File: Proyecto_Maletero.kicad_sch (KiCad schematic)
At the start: 47 parts, among them J1 DE9_Pins, J2 Conn_01x02, J3 Conn_01x02, J4 Conn_01x03, J5 Conn_01x02, J6 DE9_Pins, J8 Conn_01x02, J9 Conn_01x02, K1 FINDER-34.51, Q1 NPN, SW1 SW_Push, SW2 SW_Push, U1 LM1084-5.0, U2 MCP2551-I-SN, U3 PIC18F258-I_SO, U4 L298HN, U5 LM321, Y1 4MHz

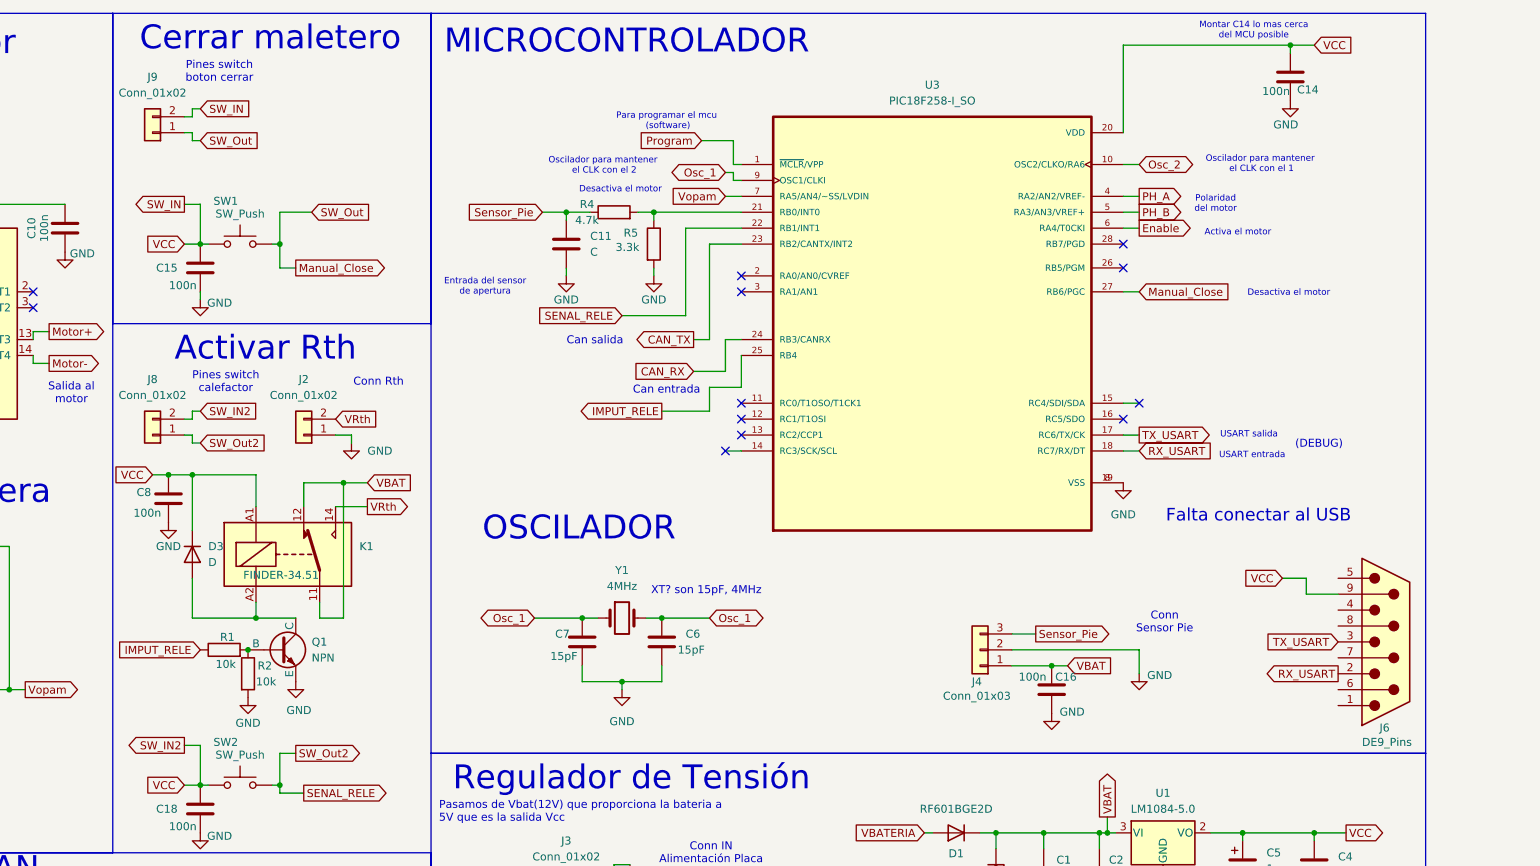
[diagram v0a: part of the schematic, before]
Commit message: Orden
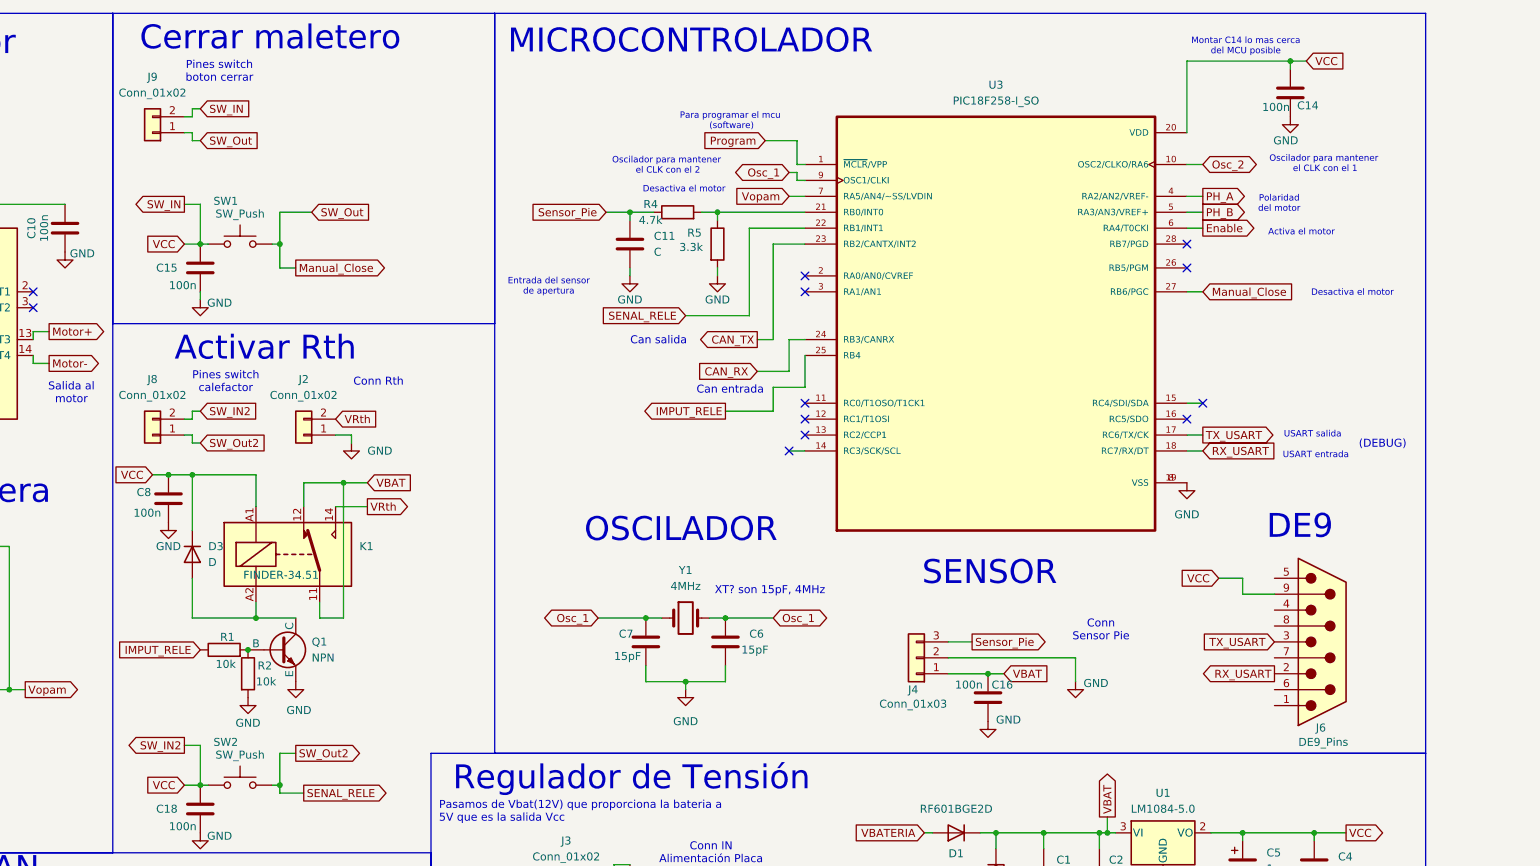
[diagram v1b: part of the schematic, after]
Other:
- note added: "DE9"
- note added: "SENSOR"
- note removed: "Falta conectar al USB"
- moved on the sheet: C11, C14, C16, C6, C7, J4, J6, R4, R5, U3, Y1
